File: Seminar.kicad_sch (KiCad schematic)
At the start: 34 parts, among them J1 USB_B_Mini, SW1 SW_Push, SW2 SW_Push, U1 NUCLEO64-F446RE, U2 PCF8574AP, U3 TPS61023DRLR, U4 TP4056

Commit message: Finito
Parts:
- D1, D2, D3, D4: Manufacturer (none) -> Vishay; Manufacturer part number (none) -> TLH540
- SW3: value ~ -> SPDT; footprint Button_Switch_SMD:Nidec_Copal_CAS-120A -> Button_Switch_THT:SW_Slide_SPDT_Straight_CK_OS102011MS2Q; Manufacturer (none) -> CAS; Manufacturer part number (none) -> CAS - 120TB1
- U3: Manufacturer (none) -> Texas Instruments; Manufacturer part number (none) -> TPS61023
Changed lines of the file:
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@@
 			)
 		)
-		(property "Datasheet" "~"
+		(property "Datasheet" "https://www.farnell.com/datasheets/2049542.pdf"
 			(at 35.56 121.92 0)
 			(effects
@@
 			)
 		)
+		(property "Manufacturer" "Vishay"
+			(at 35.56 121.92 0)
+			(effects
+				(font
+					(size 1.27 1.27)
+				)
+				(hide yes)
+			)
+		)
+		(property "Manufacturer part number" "TLH540"
+			(at 35.56 121.92 0)
+			(effects
+				(font
+					(size 1.27 1.27)
+				)
+				(hide yes)
+			)
+		)
 		(pin "1"
 		)
@@
 			)
 		)
+		(property "Manufacturer" "Texas Instruments"
+			(at 115.57 49.53 0)
+			(effects
+				(font
+					(size 1.27 1.27)
+				)
+				(hide yes)
+			)
+		)
+		(property "Manufacturer part number" "TPS61023"
+			(at 115.57 49.53 0)
+			(effects
+				(font
+					(size 1.27 1.27)
+				)
+				(hide yes)
+			)
+		)
 		(pin "2"
 		)
@@
 			)
 		)
-		(property "Datasheet" "~"
+		(property "Datasheet" "https://www.farnell.com/datasheets/2049542.pdf"
 			(at 26.67 121.92 0)
 			(effects
@@
 			)
 		)
+		(property "Manufacturer" "Vishay"
+			(at 26.67 121.92 0)
+			(effects
+				(font
+					(size 1.27 1.27)
+				)
+				(hide yes)
+			)
+		)
+		(property "Manufacturer part number" "TLH540"
+			(at 26.67 121.92 0)
+			(effects
+				(font
+					(size 1.27 1.27)
+				)
+				(hide yes)
+			)
+		)
 		(pin "2"
 		)
@@
 			)
 		)
-		(property "Datasheet" "~"
+		(property "Datasheet" "https://www.farnell.com/datasheets/2049542.pdf"
 			(at 91.44 102.87 0)
 			(effects
@@
 			)
 		)
+		(property "Manufacturer" "Vishay"
+			(at 91.44 102.87 90)
+			(effects
+				(font
+					(size 1.27 1.27)
+				)
+				(hide yes)
+			)
+		)
+		(property "Manufacturer part number" "TLH540"
+			(at 91.44 102.87 90)
+			(effects
+				(font
+					(size 1.27 1.27)
+				)
+				(hide yes)
+			)
+		)
 		(pin "2"
 		)
@@
 			)
 		)
-		(property "Datasheet" "~"
+		(property "Datasheet" "https://www.farnell.com/datasheets/2049542.pdf"
 			(at 83.82 102.87 0)
 			(effects
@@
 			)
 		)
+		(property "Manufacturer" "Vishay"
+			(at 83.82 102.87 90)
+			(effects
+				(font
+					(size 1.27 1.27)
+				)
+				(hide yes)
+			)
+		)
+		(property "Manufacturer part number" "TLH540"
+			(at 83.82 102.87 90)
+			(effects
+				(font
+					(size 1.27 1.27)
+				)
+				(hide yes)
+			)
+		)
 		(pin "2"
 		)
@@
 			)
 		)
-		(property "Value" "~"
+		(property "Value" "SPDT"
 			(at 91.44 43.18 0)
 			(effects
@@
 			)
 		)
-		(property "Footprint" "Button_Switch_SMD:Nidec_Copal_CAS-120A"
+		(property "Footprint" "Button_Switch_THT:SW_Slide_SPDT_Straight_CK_OS102011MS2Q"
 			(at 91.44 39.37 0)
 			(effects
@@
 			(at 91.44 49.53 0)
 			(effects
+				(font
+					(size 1.27 1.27)
+				)
+				(hide yes)
+			)
+		)
+		(property "Manufacturer" "CAS"
+			(at 91.44 49.53 0)
+			(effects
+				(font
+					(size 1.27 1.27)
+				)
+				(hide yes)
+			)
+		)
+		(property "Manufacturer part number" "CAS - 120TB1"
+			(at 91.44 49.53 0)
+			(effects

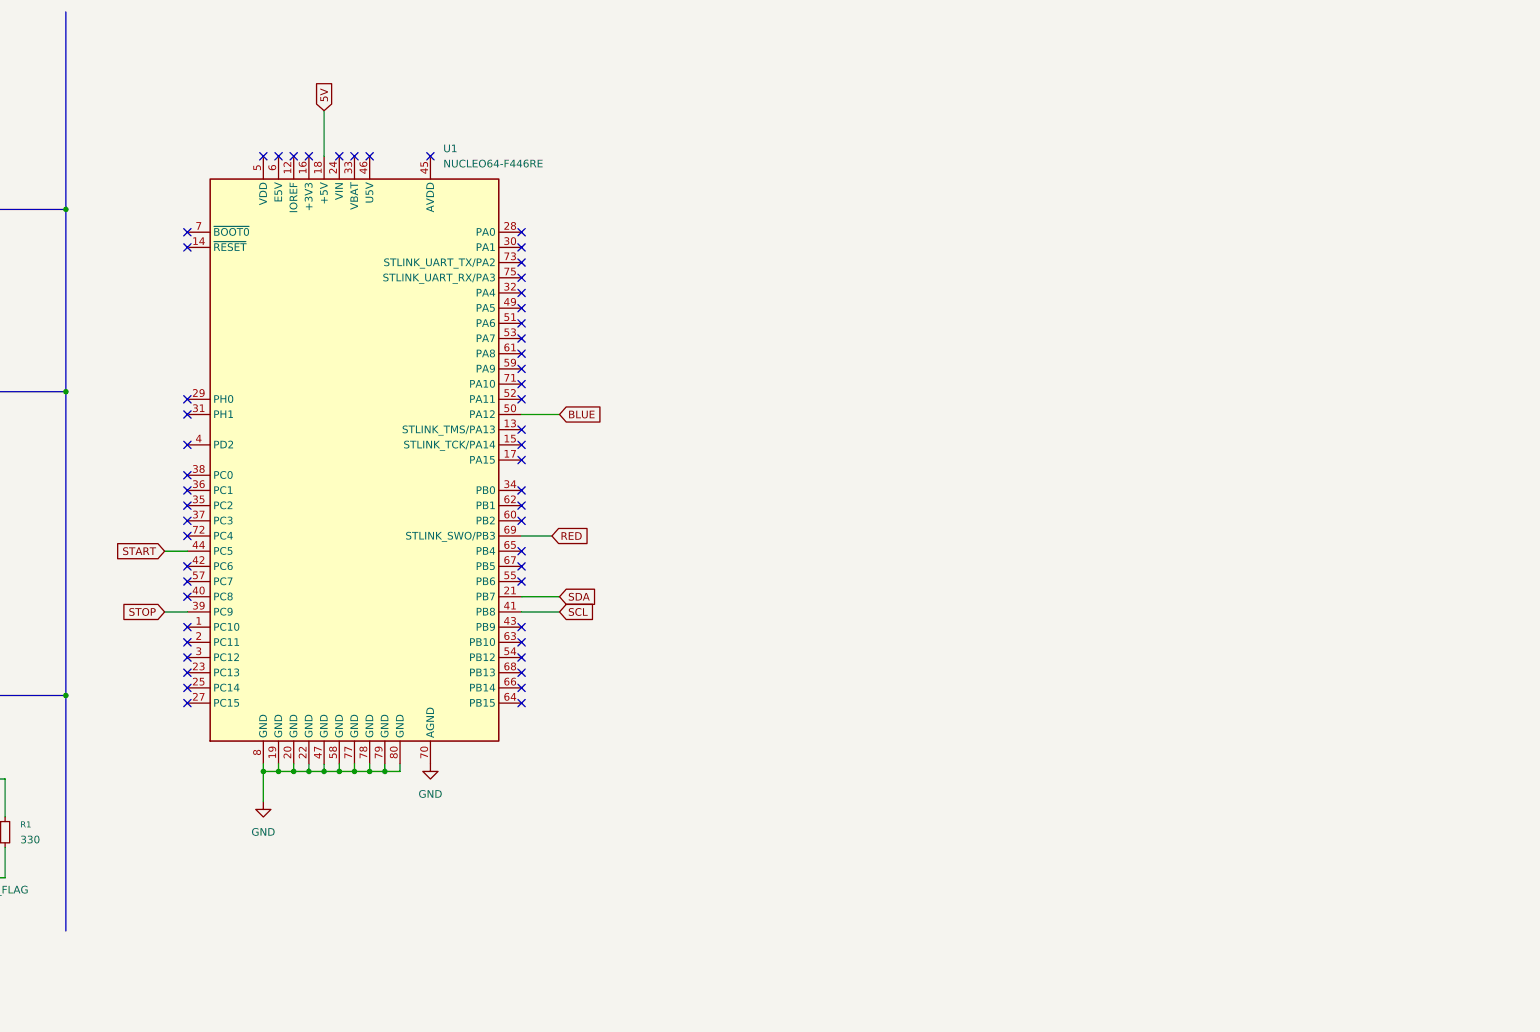
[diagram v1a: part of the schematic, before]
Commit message: PCB Update
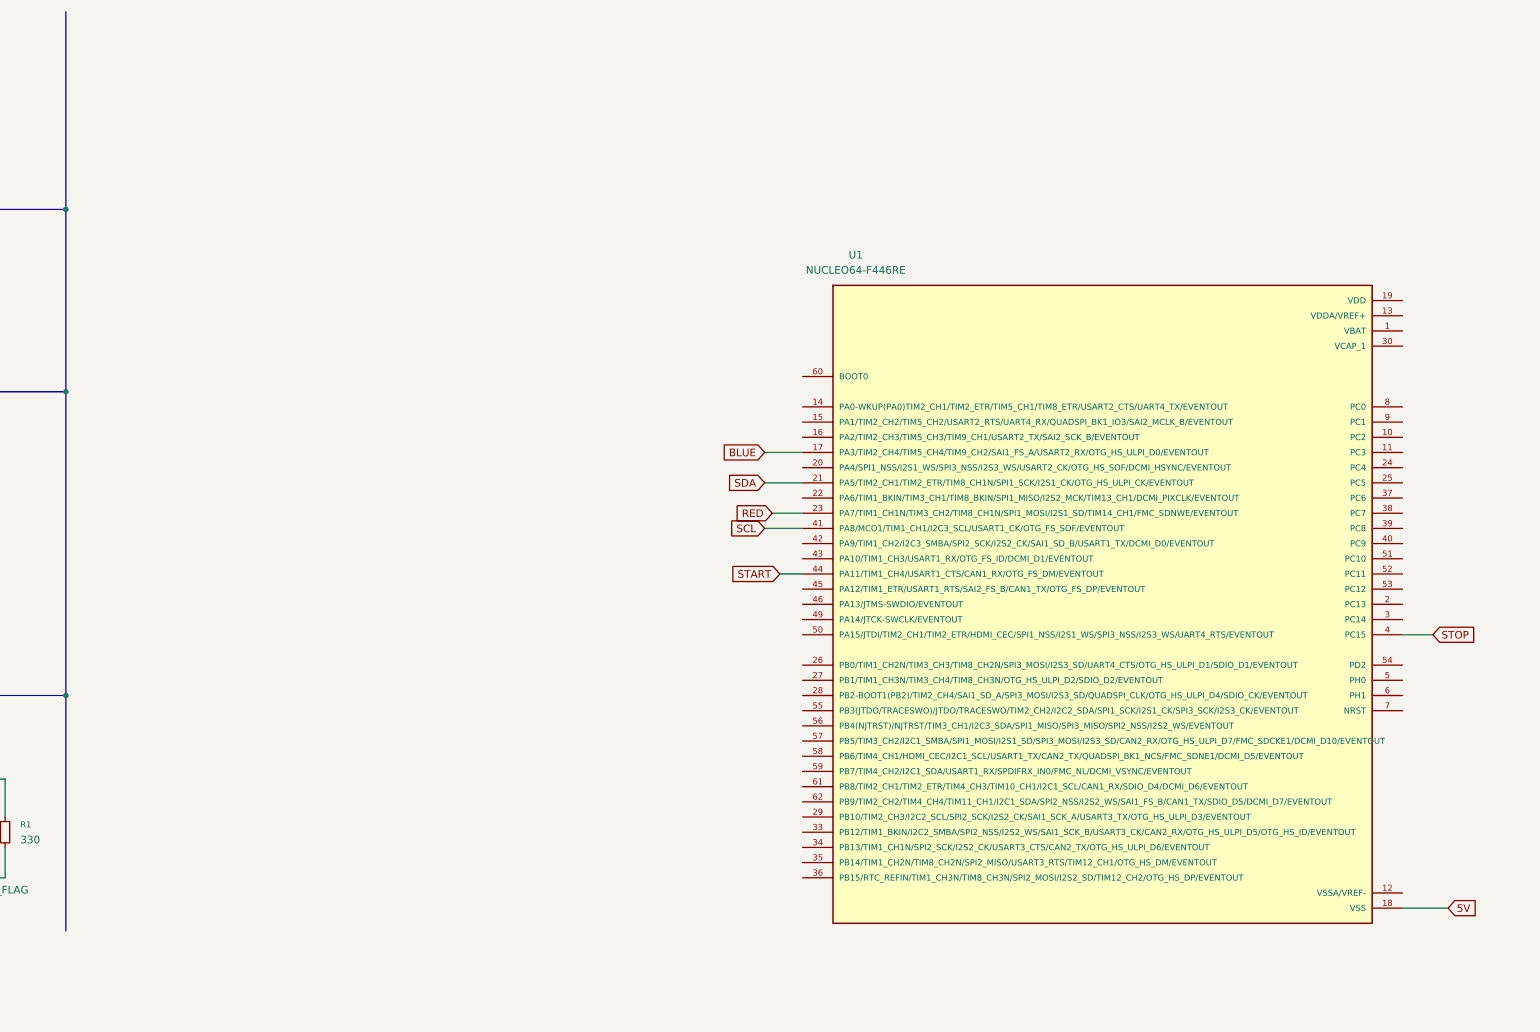
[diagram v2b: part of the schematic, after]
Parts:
- U1: footprint Module:ST_Morpho_Connector_144_STLink -> STM32F446RET6:QFP50P1200X1200X160-64N; symbol MCU_Module:NUCLEO64-F411RE -> STM32F446RET6:STM32F446RET6
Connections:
- net 5V is gone; now on net VSS: C4.1, DS1.2 (VDD), R1.1, R10.1, R4.1, R5.1, RV1.1, U1.18 (VSS), U2.16 (VDD), U3.6 (VOUT)
- net BLUE: now also U1.17 (PA3/TIM2_CH4/TIM5_CH4/TIM9_CH2/SAI1_FS_A/USART2_RX/OTG_HS_ULPI_D0/EVENTOUT); no longer U1.50 (PA12)
- net GND: no longer U1.19 (GND), U1.20 (GND), U1.22 (GND), U1.47 (GND), U1.58 (GND), U1.70 (AGND), U1.77 (GND), U1.78 (GND), U1.79 (GND), U1.8 (GND), U1.80 (GND)
- net RED: now also U1.23 (PA7/TIM1_CH1N/TIM3_CH2/TIM8_CH1N/SPI1_MOSI/I2S1_SD/TIM14_CH1/FMC_SDNWE/EVENTOUT); no longer U1.69 (STLINK_SWO/PB3)
- net STOP: now also U1.4 (PC15); no longer U1.39 (PC9)
- net VSS: now reaches U1.31 (VSS)
- net VSS: now also U1.47 (VSS), U1.63 (VSS)
- net VDD: now reaches U1.32 (VDD)
- net VDD: now also U1.19 (VDD), U1.48 (VDD), U1.64 (VDD)
- no-connect marks 63 -> 9

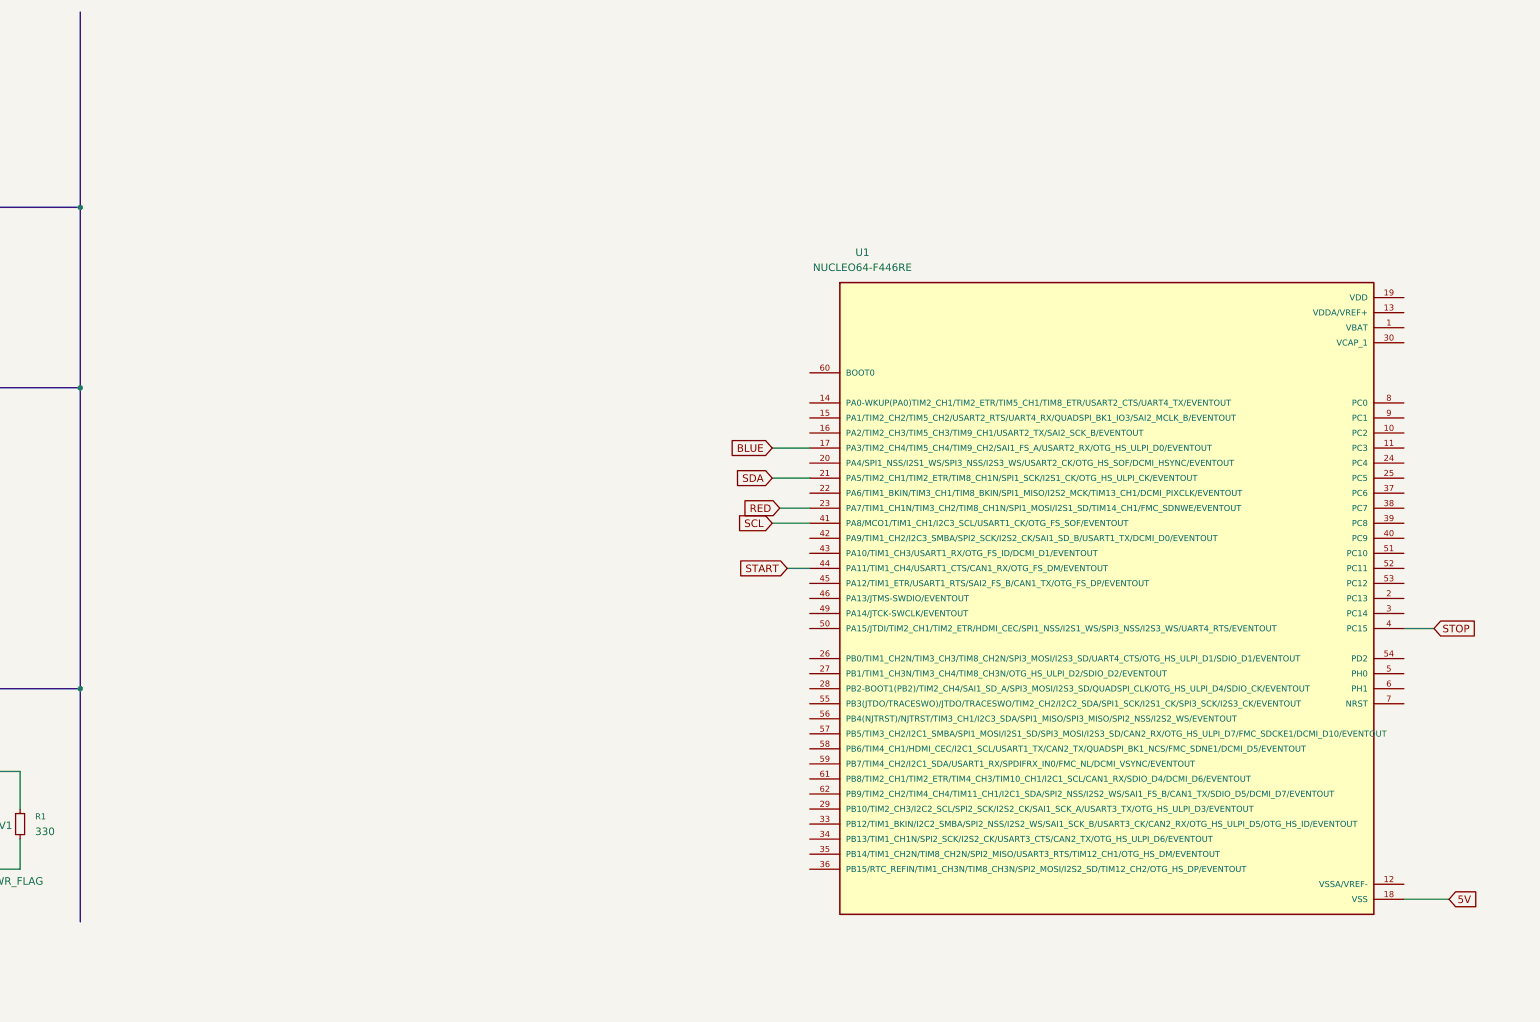
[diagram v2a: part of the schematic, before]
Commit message: a
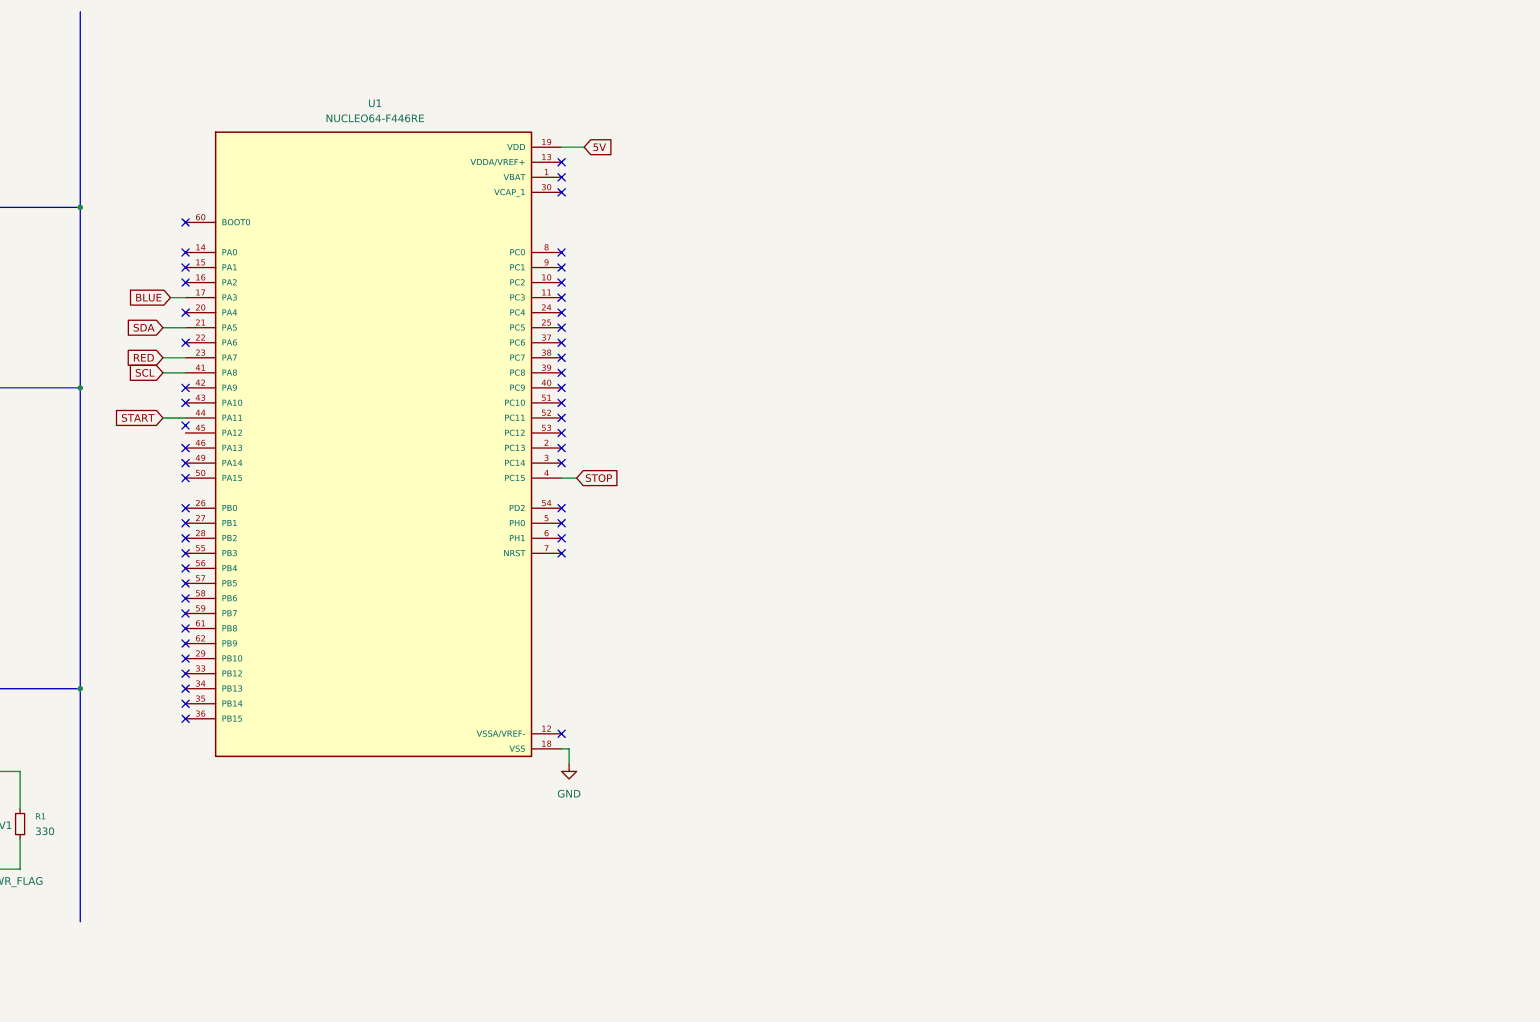
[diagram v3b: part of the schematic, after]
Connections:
- net GND: now also U1.18 (VSS), U1.31 (VSS), U1.47 (VSS), U1.63 (VSS)
- net VDD: now also C4.1, DS1.2 (VDD), R1.1, R10.1, R4.1, R5.1, RV1.1, U2.16 (VDD), U3.6 (VOUT)
- removed net VSS: C4.1, DS1.2 (VDD), R1.1, R10.1, R4.1, R5.1, RV1.1, U1.18 (VSS), U1.31 (VSS), U1.47 (VSS), U1.63 (VSS), U2.16 (VDD), U3.6 (VOUT)
- no-connect marks 9 -> 59
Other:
- moved on the sheet: U1
